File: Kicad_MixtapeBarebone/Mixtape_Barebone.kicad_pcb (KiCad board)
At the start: 2 copper layers, 34.3 x 18.4 mm, 33 parts, among them IC1 ATTINY85-20PU, J1 PB5, J10 S-Out, J11 LED, J2 PB3, J3 PB4, J4 GND, J5 PB0, J6 PB1, J7 PB2, J8 VCC, J9 Prog, SW1 SW_SPST

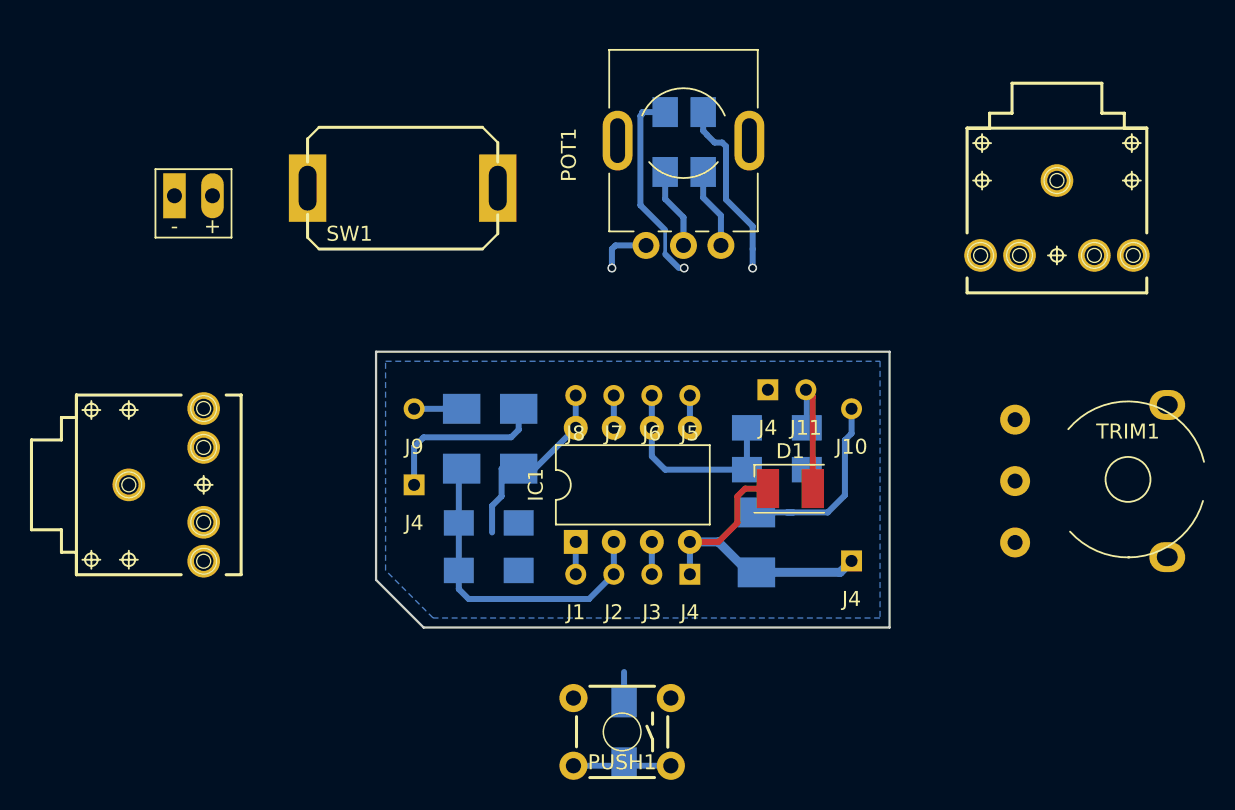
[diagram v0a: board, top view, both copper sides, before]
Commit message: Designing the MicroCore Barebone Mixtape
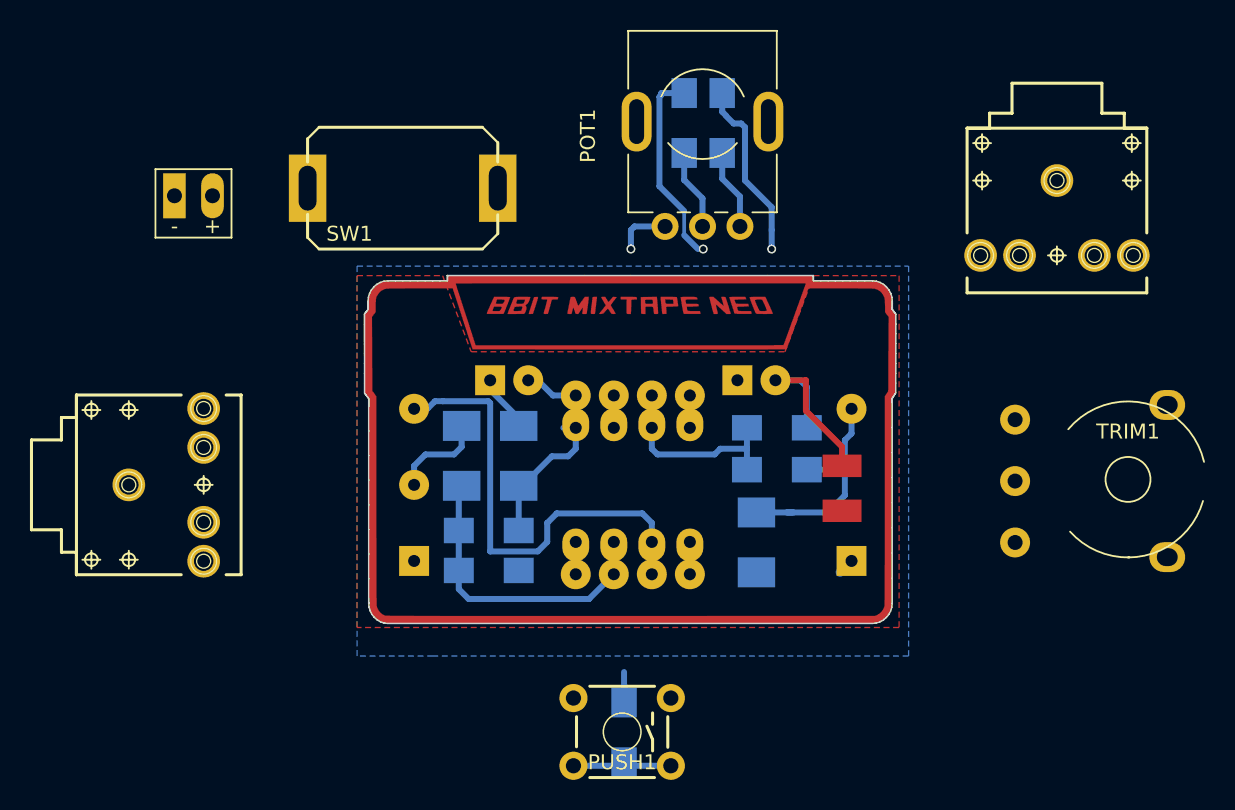
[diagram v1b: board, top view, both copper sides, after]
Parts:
- added ?: , 8BitMixtape_DIY-CAD:MicroMixtape_edge, F.Cu at (87.0, 52.1)
- added J3: PB4, 8BitMixtape_DIY-CAD:Loch_mixtape, F.Cu at (72.4, 55.9)
- added J4: GND, 8BitMixtape_DIY-CAD:GND_Loch_mixtape, F.Cu at (77.5, 54.0)
- added J8: VCC, 8BitMixtape_DIY-CAD:Loch_mixtape, F.Cu at (80.0, 54.0)
- IC1: footprint Housings_DIP:DIP-8_W7.62mm -> 8BitMixtape_DIY-CAD:Attiny_DIP-8_W7.62mm
- J1, J2, J3, J5, J6, J7, J8: footprint 8BitMixtape_DIY-CAD:Loch_mixtape -> 8BitMixtape_DIY-CAD:Loch_mixtape_seltsam
- J4: footprint 8BitMixtape_DIY-CAD:GND_Loch_mixtape -> 8BitMixtape_DIY-CAD:Loch_mixtape_seltsam
- moved J4 5.08 mm to (72.4, 66.0)
- moved J9 5.08 mm to (72.4, 61.0)
- moved D1 3.45 mm to (101.0, 61.2), turned to 90 degrees
- moved J11 2.13 mm to (96.5, 54.0)
- moved J4 2.13 mm to (94.0, 54.0)
- moved R4 1.80 mm to (90.4, 36.8)
- moved POT1 1.80 mm to (94.1, 43.7)
- moved R5 1.80 mm to (93.0, 36.8)
- moved C1 1.14 mm to (75.6, 59.0)
- moved C2 1.14 mm to (79.4, 59.0)
- moved R1 0.51 mm to (77.4, 64.0)
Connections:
- net Net-(C1-Pad1) renamed Prog
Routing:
- net Net-(IC1-Pad3): track 2.16 -> 31.5 mm
- net GND: track 38.2 -> 12.0 mm
- net Net-(D1-Pad2): track 9.36 -> 13.8 mm
- net Net-(C1-Pad2): track 3.17 -> 6.37 mm
- net VCC: track 24.8 -> 27.9 mm
- net Net-(C3-Pad2): track 12.8 -> 15.3 mm
- net Prog: track 23.6 -> 23.0 mm
- net Net-(IC1-Pad6): track 13.6 -> 13.0 mm
- added copper zone on F.Cu, net GND
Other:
- board size 34.3 x 18.4 mm -> 35.5 x 23.2 mm
